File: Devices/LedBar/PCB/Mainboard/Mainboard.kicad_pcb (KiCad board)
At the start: 2 copper layers, 63.5 x 73.7 mm, 145 parts, among them J301 12VDC/5A, J401 RS485, J501 Left, J502 Center, J503 Right, J601 0-10V(1), J701 AVR-ISP-6, Q501 Si2302DS, Q502 Si2302DS, Q503 Si2302DS, Q504 Si2302DS, Q505 Si2302DS, Q506 Si2302DS, Q507 Si2302DS, Q508 Si2302DS, Q509 Si2302DS, Q510 Si2302DS, Q511 Si2302DS, Q512 Si2302DS, Q513 Si2302DS, Q514 Si2302DS, Q515 Si2302DS, Q516 Si2302DS, SW701 button, SW702 reset, SW703 SW_DIP_x05, U301 INA219AxD, U302 AMS1117-5.0, U401 ISO3082DW, U402 B0505S-1W-SIP4, U501 PCA9685PW, U601 LM393, U701 ATmega328P-AU, U901 DS1307Z+, Y701 14.7456Mhz, Y901 23.768kHz

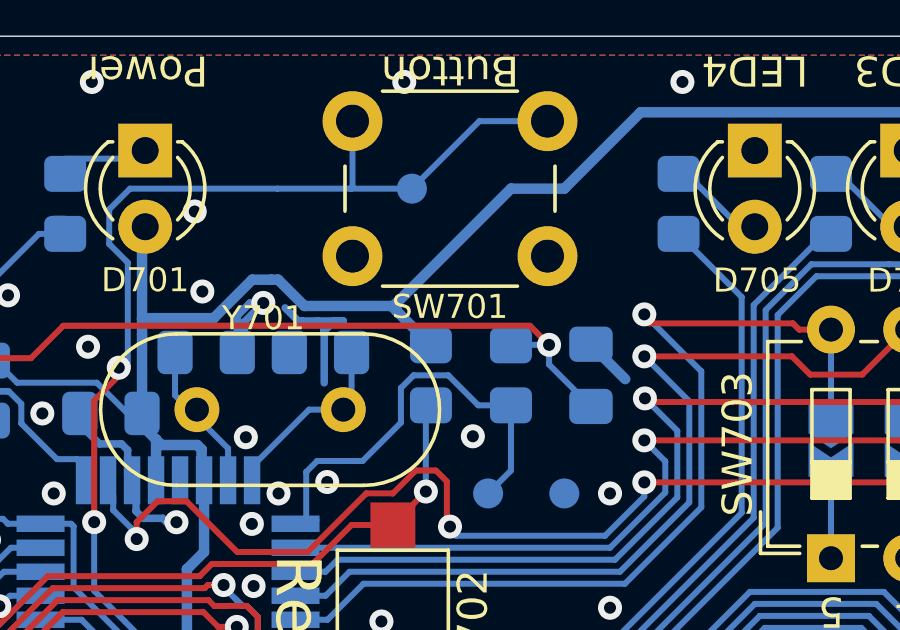
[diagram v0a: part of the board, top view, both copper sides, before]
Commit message: Working on LEDs and Button for the Case
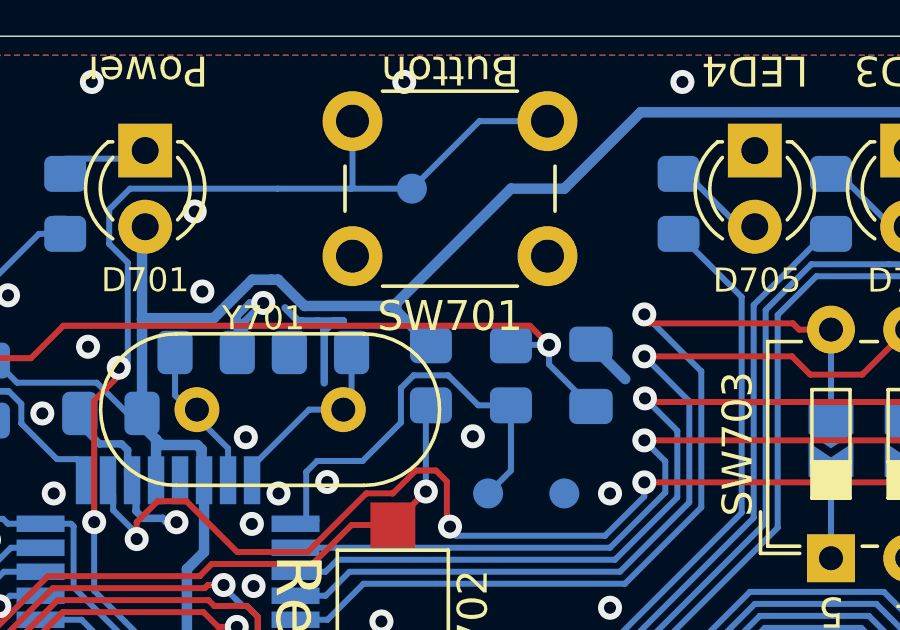
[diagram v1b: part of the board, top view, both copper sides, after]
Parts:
- SW701: footprint Button_Switch_THT:SW_PUSH_6mm_H4.3mm -> Button_Switch_THT:SW_PUSH_6mm_H8mm
